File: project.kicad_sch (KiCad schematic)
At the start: 150 parts, among them IC1 BAT5404WH6327XTSA1, J1 Conn_01x02_Pin, J2 Conn_01x02_Pin, J3 Conn_01x01_Pin, J4 Conn_01x05_Socket, J5 Conn_01x02, Q2 BSZ0902NS, Q3 BSZ0902NS, Q4 BSZ0902NS, Q5 BSZ0902NS, Q6 BSZ0902NS, Q7 BSZ0902NS, Q8 BSS138N, U1 WLC1115-68LQXQ, U2 SLS32AIA020U2USON10XTMA1, U3 LMV358AQDGKRQ1

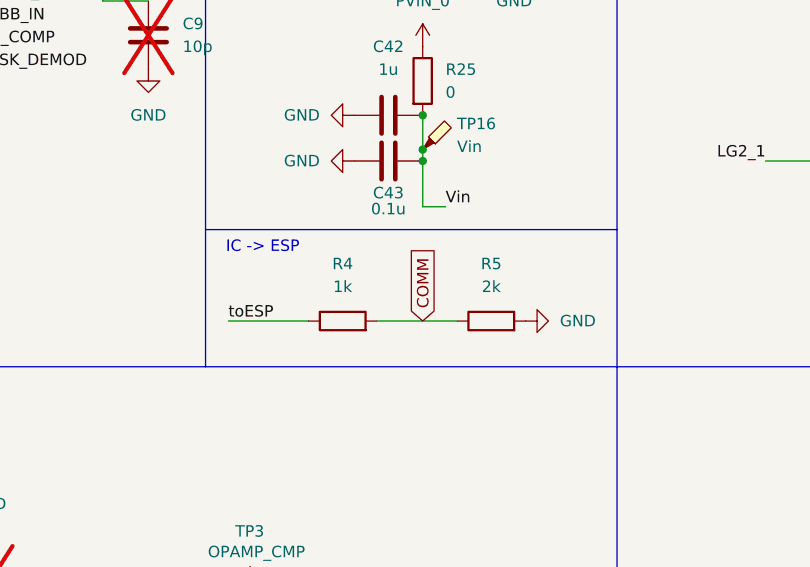
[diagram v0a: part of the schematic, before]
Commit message: before work
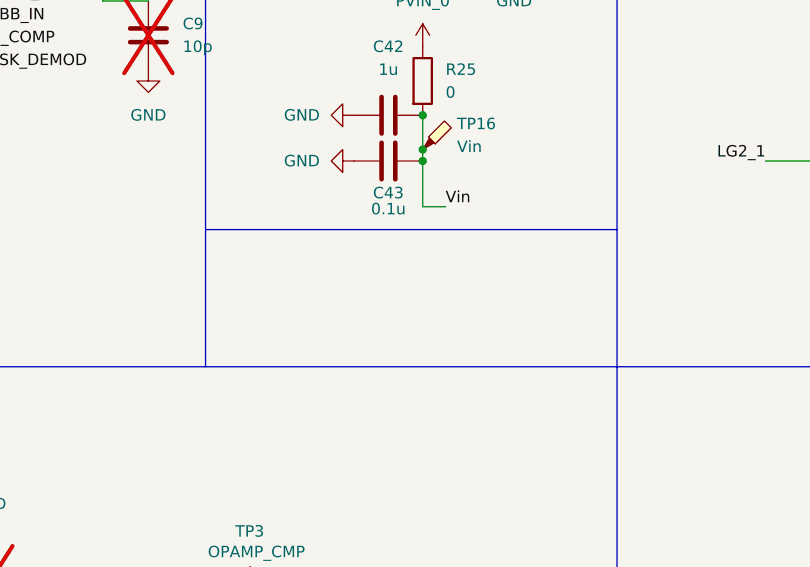
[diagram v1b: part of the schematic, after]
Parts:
- removed R4: 1k, Resistor_SMD:R_0603_1608Metric_Pad0.98x0.95mm_HandSolder, symbol Device:R
- removed R5: 2k, Resistor_SMD:R_0603_1608Metric_Pad0.98x0.95mm_HandSolder, symbol Device:R
- TP10, TP21, TP6, TP7, TP9: footprint TestPoint:TestPoint_Pad_D2.0mm -> TestPoint:TestPoint_Pad_D1.0mm
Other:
- note removed: "IC -> ESP"
